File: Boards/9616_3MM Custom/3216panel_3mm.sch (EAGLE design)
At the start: 452 parts, among them U1 74HC164D, U10 74HCT04D, U11 HT1632C, U12 HT1632C, U13 74HC164D, U14 HT1632C, U15 HT1632C, U16 74HCT04D, U17 HT1632C, U18 HT1632C, U2 HT1632C, U3 HT1632C, U4 74HCT04D, U5 HT1632C, U6 HT1632C, U7 74HC164D, U8 HT1632C, U9 HT1632C

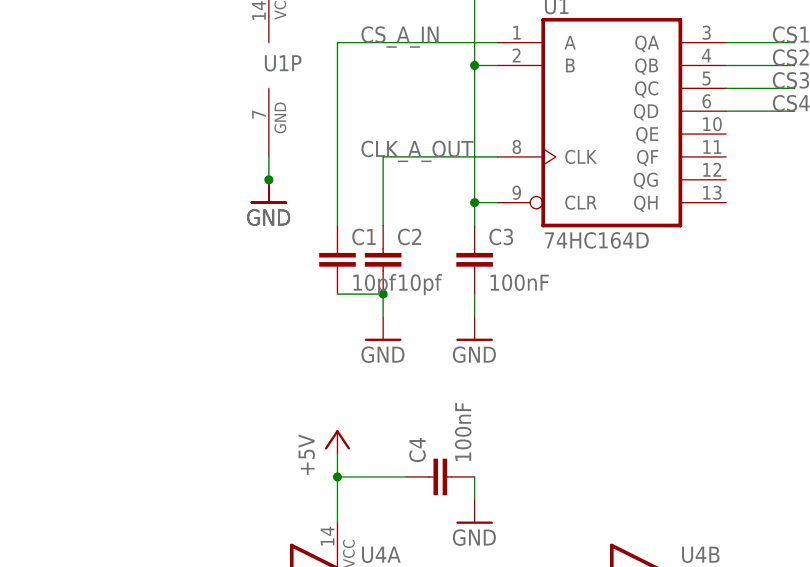
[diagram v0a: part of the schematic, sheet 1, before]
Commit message: Finished routing board (for Sierra Circuits/PCBCart.com specs)
Signed-off-by: Evan Richardson <erichardson@savi.com>
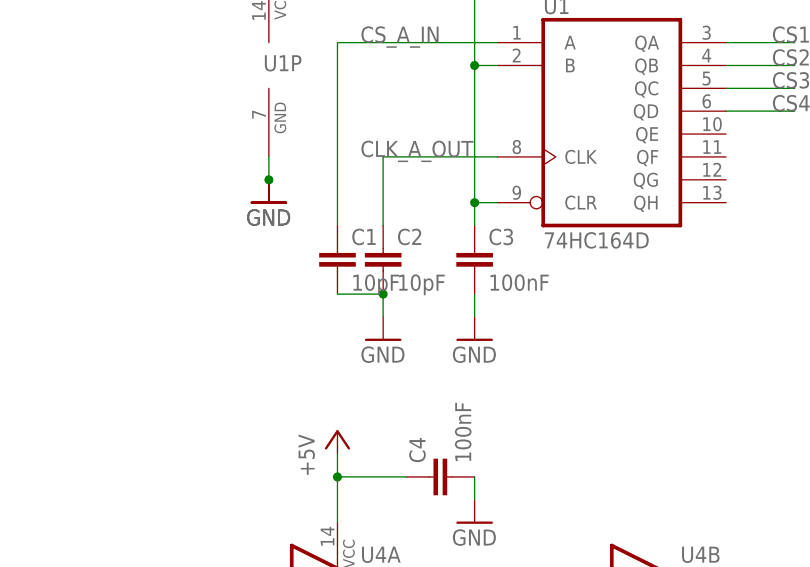
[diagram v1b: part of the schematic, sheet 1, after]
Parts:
- C1, C2: value 10pf -> 10pF
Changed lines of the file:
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@@
 <?xml version="1.0" encoding="utf-8"?>
 <!DOCTYPE eagle SYSTEM "eagle.dtd">
-<eagle version="6.0">
+<eagle version="6.1">
 <drawing>
 <settings>
@@
 </variantdefs>
 <classes>
-<class number="0" name="default" width="0.2" drill="0.2">
-<clearance class="0" value="0.2"/>
+<class number="0" name="default" width="0.254" drill="0.254">
+<clearance class="0" value="0.3048"/>
 </class>
-<class number="1" name="+5V" width="0.3048" drill="0.2">
-<clearance class="1" value="0.2"/>
+<class number="1" name="+5V" width="0.3556" drill="0.254">
+<clearance class="1" value="0.3048"/>
+</class>
+<class number="2" name="GND" width="0.3048" drill="0.254">
+<clearance class="2" value="0.3048"/>
 </class>
 </classes>
@@
 <part name="GND7" library="supply1" deviceset="GND" device=""/>
 <part name="GND8" library="supply1" deviceset="GND" device=""/>
-<part name="C2" library="SparkFun" deviceset="CAP" device="0805" value="10pf"/>
+<part name="C2" library="SparkFun" deviceset="CAP" device="0805" value="10pF"/>
 <part name="GND9" library="supply1" deviceset="GND" device=""/>
-<part name="C1" library="SparkFun" deviceset="CAP" device="0805" value="10pf"/>
+<part name="C1" library="SparkFun" deviceset="CAP" device="0805" value="10pF"/>
 <part name="P+5" library="supply1" deviceset="+5V" device=""/>
 <part name="C4" library="SparkFun" deviceset="CAP" device="0805" value="100nF"/>
@@
 </segment>
 </net>
-<net name="GND" class="0">
+<net name="GND" class="2">
 <segment>
 <pinref part="U2" gate="G$1" pin="VSS"/>
@@
 </segment>
 </net>
-<net name="GND" class="0">
+<net name="GND" class="2">
 <segment>
 <pinref part="U9" gate="G$1" pin="VSS"/>
@@
 </busses>
 <nets>
-<net name="GND" class="0">
+<net name="GND" class="2">
 <segment>
 <pinref part="U15" gate="G$1" pin="VSS"/>
